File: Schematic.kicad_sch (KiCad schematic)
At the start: 72 parts, among them J1 Screw_Terminal_01x04, J20 T44007, J21 T44007, Q1 HY1707, Q20 BC817, Q21 SUD50P06-15, U1 UC3845, U20 TCMT1108, U21 TL431M

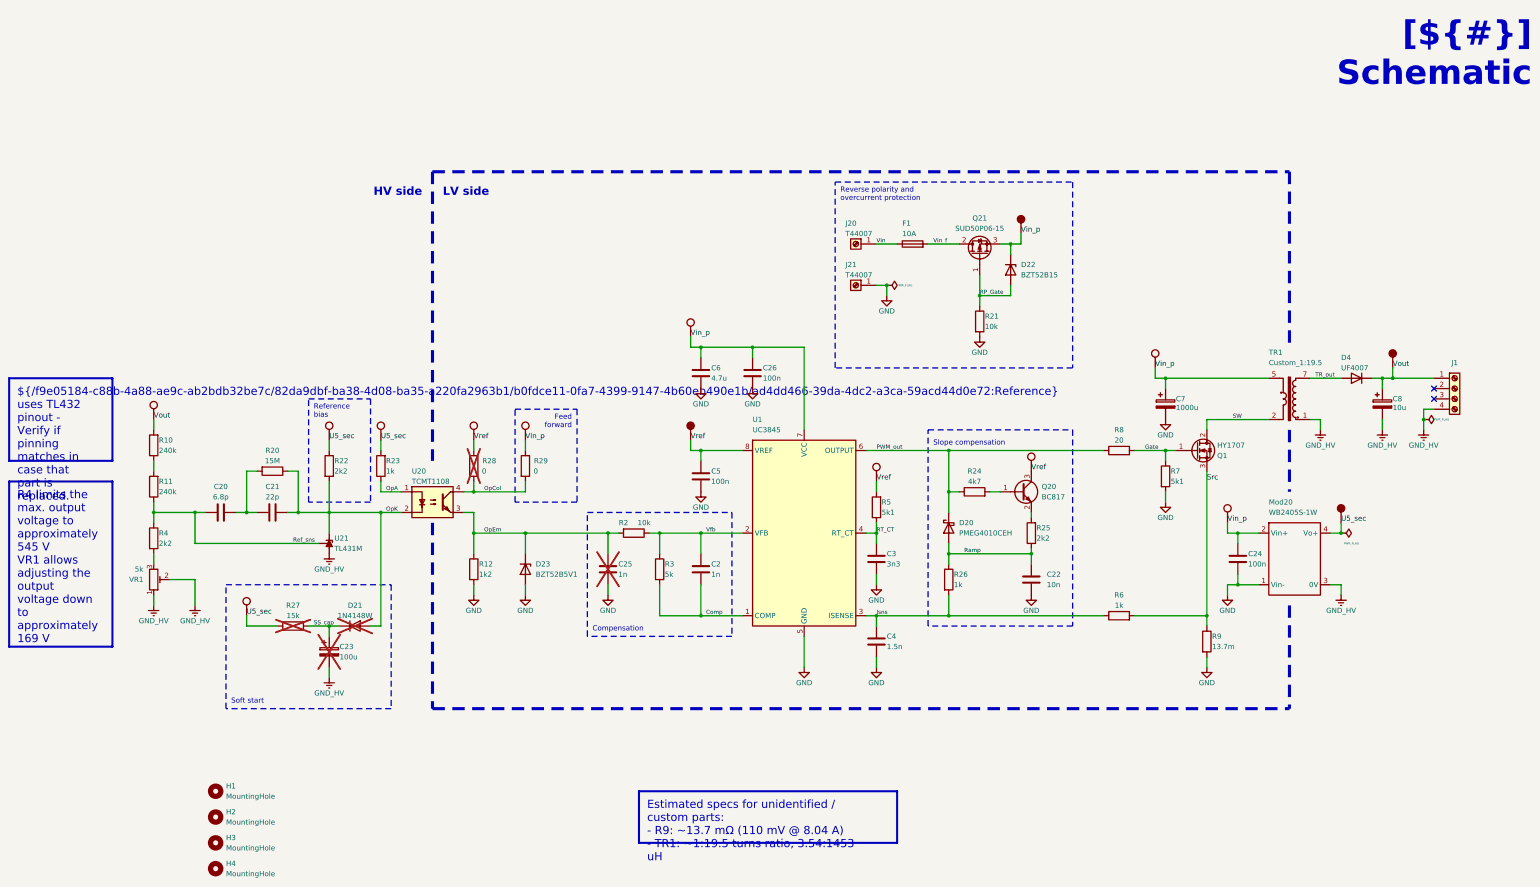
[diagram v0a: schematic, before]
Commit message: Layout candidate #2 (draft)
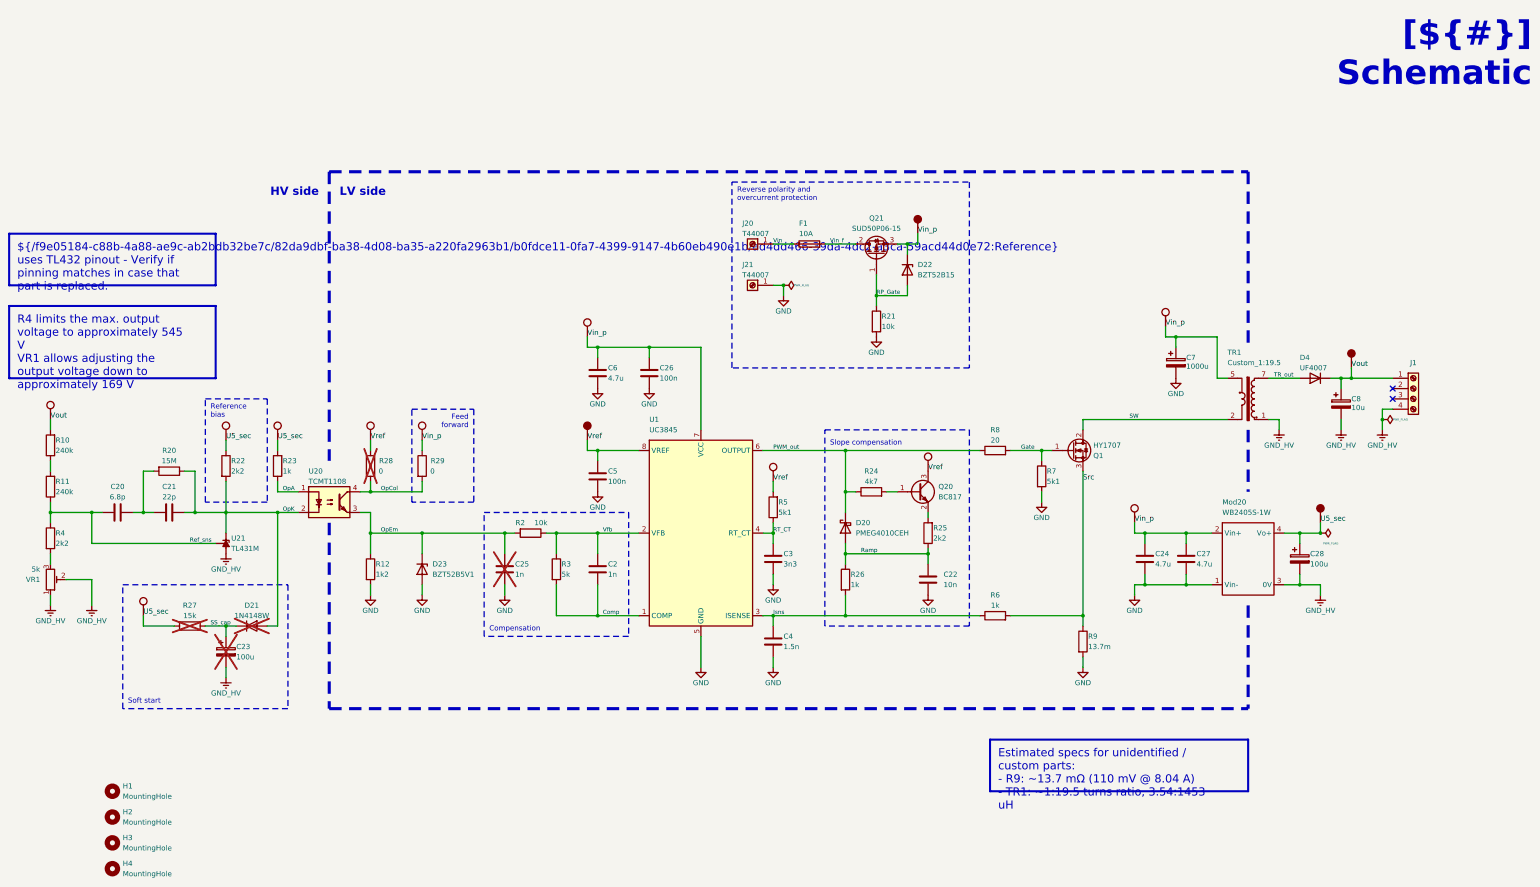
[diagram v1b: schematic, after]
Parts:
- added C27: 4.7u, Capacitor_SMD:C_0805_2012Metric_Pad1.18x1.45mm_HandSolder, symbol Device:C
- added C28: 100u, Capacitor_THT:CP_Radial_D6.3mm_P2.50mm, symbol Device:C_Polarized
- C23: footprint Capacitor_THT:CP_Radial_D8.0mm_P2.50mm -> Capacitor_THT:CP_Radial_D6.3mm_P2.50mm
- C24: value 100n -> 4.7u; footprint Capacitor_SMD:C_0603_1608Metric_Pad1.08x0.95mm_HandSolder -> Capacitor_SMD:C_0805_2012Metric_Pad1.18x1.45mm_HandSolder
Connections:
- net GND: now also C27.2
- net GND_HV: now also C28.2
- net U5_sec: now also C28.1
- net Vin_p: now also C27.1
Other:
- moved on the sheet: C2, C20, C21, C22, C23, C25, C26, C3, C4, C5, C6, C7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
